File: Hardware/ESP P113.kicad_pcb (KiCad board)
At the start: 2 copper layers, 104.8 x 73.7 mm, 55 parts, among them J1 L_In, J2 R_In, J3 L_Out, J4 R_Out, J5 AC_In, Q1 MJE15032, Q2 MJE15033, Q3 MJE15032, Q4 MJE15033, U1 LM4562

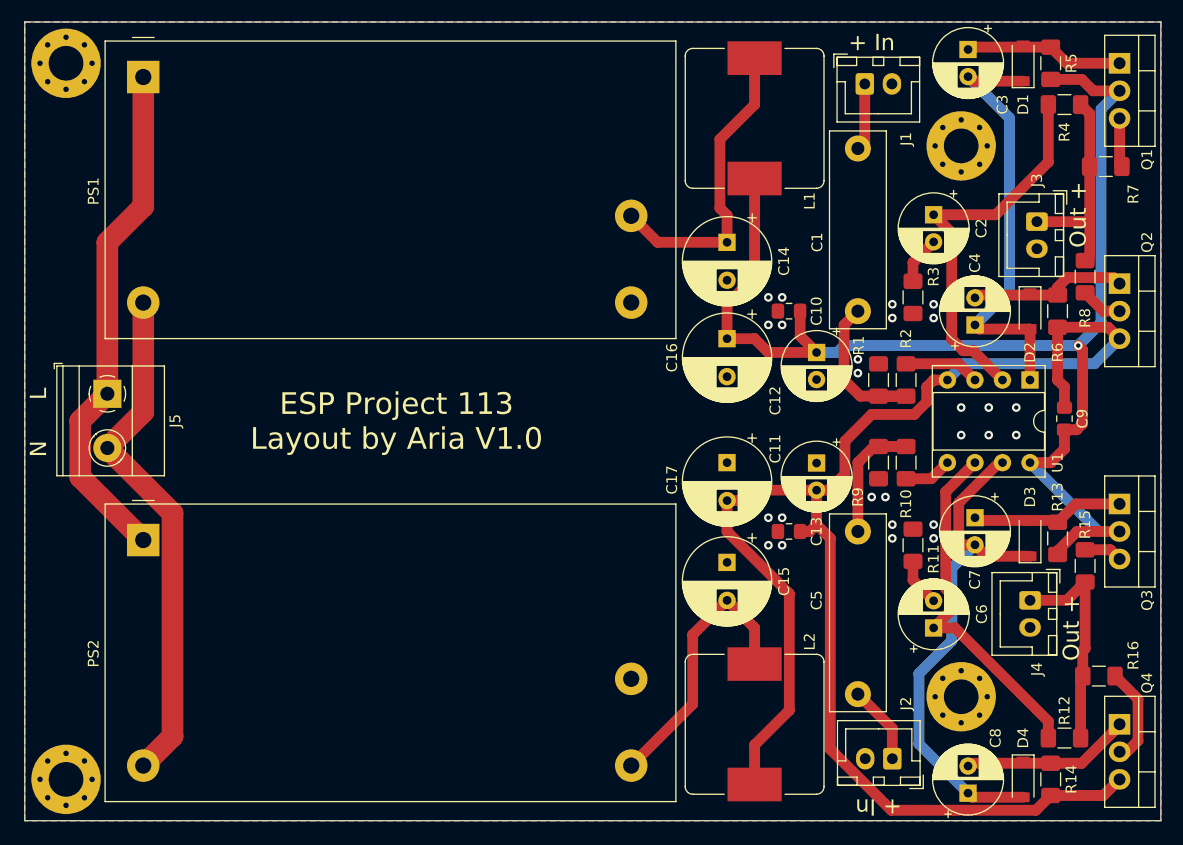
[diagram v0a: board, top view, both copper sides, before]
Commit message: Updated to V1.1
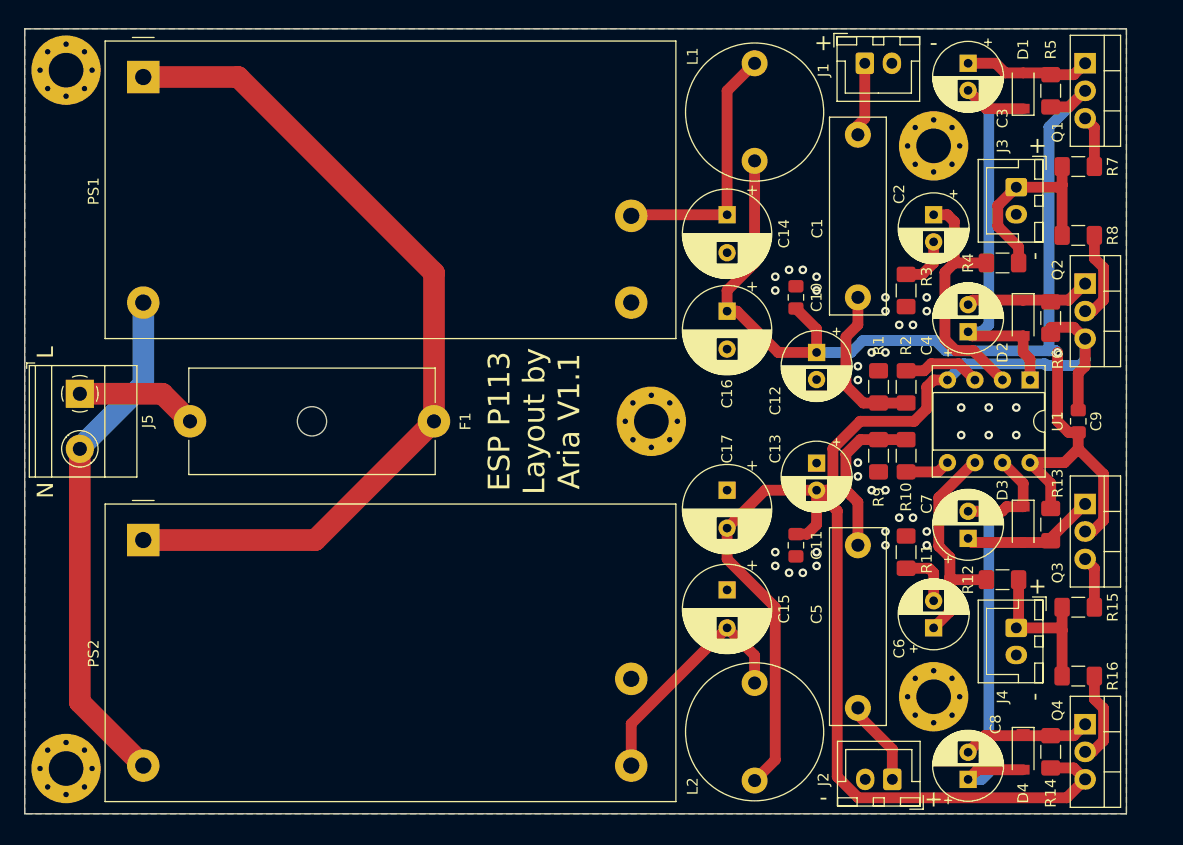
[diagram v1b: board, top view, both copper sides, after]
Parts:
- added F1: Fuse_Small, Fuse:Fuseholder_Cylinder-5x20mm_Schurter_0031_8201_Horizontal_Open, F.Cu at (74.9, 62.2)
- added H5: MountingHole, MountingHole:MountingHole_3.2mm_M3_Pad_Via, F.Cu at (63.5, 29.8)
- J5: footprint TerminalBlock_Phoenix:TerminalBlock_Phoenix_MKDS-1,5-2_1x02_P5.00mm_Horizontal -> TerminalBlock_Phoenix:TerminalBlock_Phoenix_MKDS-1,5-2-5.08_1x02_P5.08mm_Horizontal
- L1, L2: footprint Inductor_SMD:L_Bourns_SRP1245A -> Inductor_THT:L_Radial_D12.5mm_P9.00mm_Fastron_09HCP
- moved H1 63.3 mm to (117.5, 62.2)
- moved R12 15.7 mm to (149.9, 76.8)
- moved R4 15.7 mm to (149.9, 47.6)
- moved L1 5.08 mm to (127.0, 29.2)
- moved R15 3.86 mm to (156.8, 79.4), turned to 180 degrees
- moved R8 3.86 mm to (156.8, 45.1), turned to 0 degrees
- moved L2 3.81 mm to (127.0, 86.4)
- moved J3 3.70 mm to (151.1, 40.6)
- moved Q1 3.18 mm to (157.5, 29.2)
- moved Q2 3.18 mm to (157.5, 49.5)
- moved Q3 3.18 mm to (157.5, 69.8)
- moved Q4 3.18 mm to (157.5, 90.2)
- moved J4 2.84 mm to (151.1, 81.3)
- moved H3 2.54 mm to (143.5, 36.8)
- moved H4 2.54 mm to (143.5, 87.6)
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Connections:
- J5 pad 1: Net-(J5-Pad1) -> Net-(F1-Pad1)
- PS1 pad 1: Net-(J5-Pad1) -> Net-(F1-Pad2)
- PS2 pad 1: Net-(J5-Pad1) -> Net-(F1-Pad2)
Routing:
- net Net-(F1-Pad2): track 0.00 -> 79.3 mm
- net Net-(J5-Pad1): track 47.5 -> 0.00 mm
- net Net-(C2-Pad1): track 36.3 -> 23.2 mm
- net Net-(F1-Pad1): track 0.00 -> 11.2 mm
- net Net-(C6-Pad1): track 32.8 -> 24.4 mm
- net +15: track 117.7 -> 111.1 mm
- net R_Out: track 20.3 -> 15.2 mm
- net Net-(C7-Pad2): track 48.4 -> 43.3 mm
- net Net-(Q2-Pad2): track 3.87 -> 8.43 mm
- net Net-(C14-Pad1): track 28.4 -> 23.9 mm
- net Net-(C8-Pad2): track 15.6 -> 11.9 mm
- net -15: track 145.3 -> 141.8 mm
- net Net-(C15-Pad2): track 26.4 -> 23.1 mm
- net Net-(C3-Pad2): track 43.1 -> 39.9 mm
- net Net-(C4-Pad2): track 14.8 -> 11.6 mm
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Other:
- board size 104.8 x 73.7 mm -> 101.6 x 72.4 mm
- board text added: "+"
- board text added: "-"
- board text added: "ESP P113 Layout by Aria V1.1"
- board text removed: "+ In"
- board text removed: "ESP Project 113 Layout by Aria V1.0"
- board text removed: "Out +"
